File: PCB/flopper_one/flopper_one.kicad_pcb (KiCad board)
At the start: 2 copper layers, 76.8 x 63 mm, 24 parts, among them J1 To PN532 ->, J2 <- ST7789, Q1 2N2219, SW1 SW_Omron_B3FS, SW2 SW_Omron_B3FS, SW3 SW_Omron_B3FS, SW4 SW_Omron_B3FS, SW5 SW_Omron_B3FS, SW6 SW_SPST, U1 TP4056-42-ESOP8, U4 hw-045

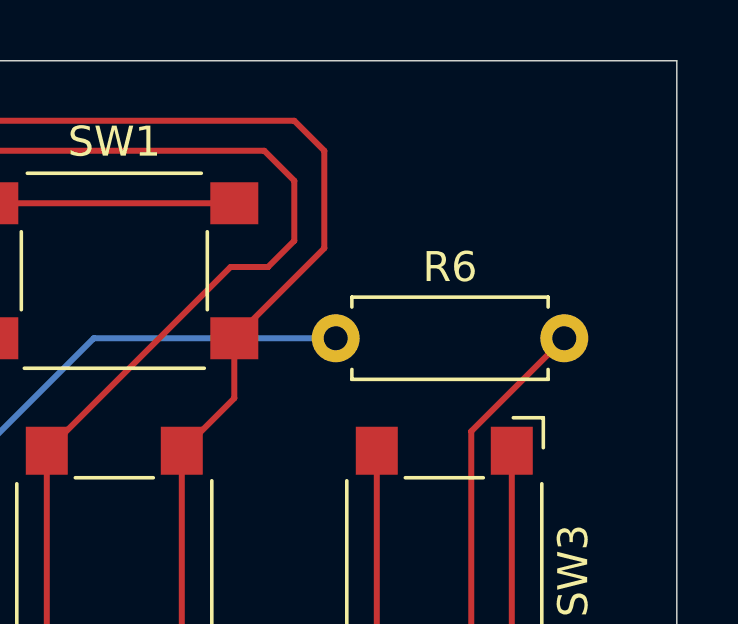
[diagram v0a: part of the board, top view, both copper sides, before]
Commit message: flip r6
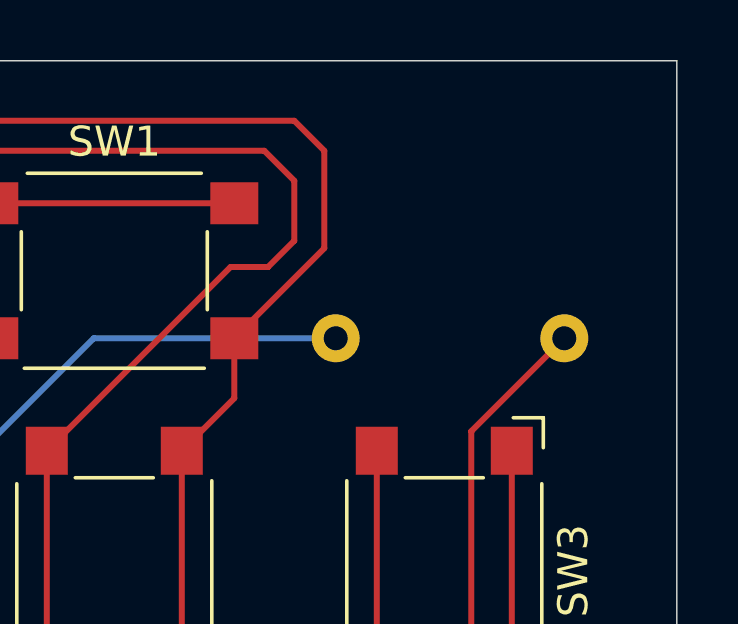
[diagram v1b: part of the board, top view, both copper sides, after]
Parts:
- R6: moved to B.Cu
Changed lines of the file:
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@@
-		)
-	)
-	(footprint "Resistor_THT:R_Axial_DIN0207_L6.3mm_D2.5mm_P7.62mm_Horizontal"
-		(layer "F.Cu")
-		(at 98.38 33.5)
-		(descr "Resistor, Axial_DIN0207 series, Axial, Horizontal, pin pitch=7.62mm, 0.25W = 1/4W, length*diameter=6.3*2.5mm^2, http://cdn-reichelt.de/documents/datenblatt/B400/1_4W%23YAG.pdf")
-		(tags "Resistor Axial_DIN0207 series Axial Horizontal pin pitch 7.62mm 0.25W = 1/4W length 6.3mm diameter 2.5mm")
-		(property "Reference" "R6"
-			(at 3.81 -2.37 0)
-			(layer "F.SilkS")
-			(effects
-				(font
-					(size 1 1)
-					(thickness 0.15)
-				)
-			)
-		)
-		(property "Value" "0.4Ω"
-			(at 3.81 2.37 0)
-			(layer "F.Fab")
-			(effects
-				(font
-					(size 1 1)
-					(thickness 0.15)
-				)
-			)
-		)
-		(property "Datasheet" "~"
-			(at 0 0 0)
-			(layer "F.Fab")
-			(hide yes)
-			(effects
-				(font
-					(size 1.27 1.27)
-					(thickness 0.15)
-				)
-			)
-		)
-		(property "Description" "Resistor, US symbol"
-			(at 0 0 0)
-			(layer "F.Fab")
-			(hide yes)
-			(effects
-				(font
-					(size 1.27 1.27)
-					(thickness 0.15)
-				)
-			)
-		)
-		(property ki_fp_filters "R_*")
-		(sheetname "/")
-		(sheetfile "flopper_one.kicad_sch")
-		(attr through_hole)
-		(fp_line
-			(start 0.54 -1.37)
-			(end 7.08 -1.37)
-			(stroke
-				(width 0.12)
-				(type solid)
-			)
-			(layer "F.SilkS")
-		)
-		(fp_line
-			(start 0.54 -1.04)
-			(end 0.54 -1.37)
-			(stroke
-				(width 0.12)
-				(type solid)
-			)
-			(layer "F.SilkS")
-		)
-		(fp_line
-			(start 0.54 1.04)
-			(end 0.54 1.37)
-			(stroke
-				(width 0.12)
-				(type solid)
-			)
-			(layer "F.SilkS")
-		)
-		(fp_line
-			(start 0.54 1.37)
-			(end 7.08 1.37)
-			(stroke
-				(width 0.12)
-				(type solid)
-			)
-			(layer "F.SilkS")
-		)
-		(fp_line
-			(start 7.08 -1.37)
-			(end 7.08 -1.04)
-			(stroke
-				(width 0.12)
-				(type solid)
-			)
-			(layer "F.SilkS")
-		)
-		(fp_line
-			(start 7.08 1.37)
-			(end 7.08 1.04)
-			(stroke
-				(width 0.12)
-				(type solid)
-			)
-			(layer "F.SilkS")
-		)
-		(fp_rect
-			(start -1.05 -1.5)
-			(end 8.67 1.5)
-			(stroke
-				(width 0.05)
-				(type solid)
-			)
-			(fill no)
-			(layer "F.CrtYd")
-		)
-		(fp_line
-			(start 0 0)
-			(end 0.66 0)
-			(stroke
-				(width 0.1)
-				(type solid)
-			)
-			(layer "F.Fab")
-		)
-		(fp_line
-			(start 7.62 0)
-			(end 6.96 0)
-			(stroke
-				(width 0.1)
-				(type solid)
-			)
-			(layer "F.Fab")
-		)
-		(fp_rect
-			(start 0.66 -1.25)
-			(end 6.96 1.25)
-			(stroke
-				(width 0.1)
-				(type solid)
-			)
-			(fill no)
-			(layer "F.Fab")
-		)
-		(fp_text user "${REFERENCE}"
-			(at 3.81 0 0)
-			(layer "F.Fab")
-			(effects
-				(font
-					(size 1 1)
-					(thickness 0.15)
-				)
-			)
-		)
-		(pad "1" thru_hole circle
-			(at 0 0)
-			(size 1.6 1.6)
-			(drill 0.8)
-			(layers "*.Cu" "*.Mask")
-			(remove_unused_layers no)
-			(net 40 "/VIN")
-			(pintype "passive")
-		)
-		(pad "2" thru_hole circle
-			(at 7.62 0)
-			(size 1.6 1.6)
-			(drill 0.8)
-			(layers "*.Cu" "*.Mask")
-			(remove_unused_layers no)
-			(net 42 "Net-(D2-A)")
-			(pintype "passive")
-		)
-		(embedded_fonts no)
-		(model "${KICAD9_3DMODEL_DIR}/Resistor_THT.3dshapes/R_Axial_DIN0207_L6.3mm_D2.5mm_P7.62mm_Horizontal.step"
-			(offset
-				(xyz 0 0 0)
-			)
-			(scale
-				(xyz 1 1 1)
-			)
-			(rotate
-				(xyz 0 0 0)
-			)
 		)
 	)
@@
 			(offset
 				(xyz 0 0 0)
+			)
+			(scale
+				(xyz 1 1 1)
+			)
+			(rotate
+				(xyz 0 0 0)
+			)
+		)
+	)
+	(footprint "Resistor_THT:R_Axial_DIN0207_L6.3mm_D2.5mm_P7.62mm_Horizontal"
+		(layer "B.Cu")
+		(at 98.38 33.5)
+		(descr "Resistor, Axial_DIN0207 series, Axial, Horizontal, pin pitch=7.62mm, 0.25W = 1/4W, length*diameter=6.3*2.5mm^2, http://cdn-reichelt.de/documents/datenblatt/B400/1_4W%23YAG.pdf")
+		(tags "Resistor Axial_DIN0207 series Axial Horizontal pin pitch 7.62mm 0.25W = 1/4W length 6.3mm diameter 2.5mm")
+		(property "Reference" "R6"
+			(at 3.81 2.37 0)
+			(layer "B.SilkS")
+			(effects
+				(font
+					(size 1 1)
+					(thickness 0.15)
+				)
+				(justify mirror)
+			)
+		)
+		(property "Value" "0.4Ω"
+			(at 3.81 -2.37 0)
+			(layer "B.Fab")
+			(effects
+				(font
+					(size 1 1)
+					(thickness 0.15)
+				)
+				(justify mirror)
+			)
+		)
+		(property "Datasheet" "~"
+			(at 0 0 0)
+			(layer "B.Fab")
+			(hide yes)
+			(effects
+				(font
+					(size 1.27 1.27)
+					(thickness 0.15)
+				)
+				(justify mirror)
+			)
+		)
+		(property "Description" "Resistor, US symbol"
+			(at 0 0 0)
+			(layer "B.Fab")
+			(hide yes)
+			(effects
+				(font
+					(size 1.27 1.27)
+					(thickness 0.15)
+				)
+				(justify mirror)
+			)
+		)
+		(property ki_fp_filters "R_*")
+		(sheetname "/")
+		(sheetfile "flopper_one.kicad_sch")
+		(attr through_hole)
+		(fp_line
+			(start 0.54 -1.37)
+			(end 7.08 -1.37)
+			(stroke
+				(width 0.12)
+				(type solid)
+			)
+			(layer "B.SilkS")
+		)
+		(fp_line
+			(start 0.54 -1.04)
+			(end 0.54 -1.37)
+			(stroke
+				(width 0.12)
+				(type solid)
+			)
+			(layer "B.SilkS")
+		)
+		(fp_line
+			(start 0.54 1.04)
+			(end 0.54 1.37)
+			(stroke
+				(width 0.12)
+				(type solid)
+			)
+			(layer "B.SilkS")
+		)
+		(fp_line
+			(start 0.54 1.37)
+			(end 7.08 1.37)
+			(stroke
+				(width 0.12)
+				(type solid)
+			)
+			(layer "B.SilkS")
+		)
+		(fp_line
+			(start 7.08 -1.37)
+			(end 7.08 -1.04)
+			(stroke
+				(width 0.12)
+				(type solid)
+			)
+			(layer "B.SilkS")
+		)
+		(fp_line
+			(start 7.08 1.37)
+			(end 7.08 1.04)
+			(stroke
+				(width 0.12)
+				(type solid)
+			)
+			(layer "B.SilkS")
+		)
+		(fp_rect
+			(start -1.05 1.5)
+			(end 8.67 -1.5)
+			(stroke
+				(width 0.05)
+				(type solid)
+			)
+			(fill no)
+			(layer "B.CrtYd")
+		)
+		(fp_line
+			(start 0 0)
+			(end 0.66 0)
+			(stroke
+				(width 0.1)
+				(type solid)
+			)
+			(layer "B.Fab")
+		)
+		(fp_line
+			(start 7.62 0)
+			(end 6.96 0)
+			(stroke
+				(width 0.1)
+				(type solid)
+			)
+			(layer "B.Fab")
+		)
+		(fp_rect
+			(start 0.66 1.25)
+			(end 6.96 -1.25)
+			(stroke
+				(width 0.1)
+				(type solid)
+			)
+			(fill no)
+			(layer "B.Fab")
+		)
+		(fp_text user "${REFERENCE}"
+			(at 3.81 0 0)
+			(layer "B.Fab")
+			(effects
+				(font
+					(size 1 1)
+					(thickness 0.15)
+				)
+				(justify mirror)
+			)
+		)
+		(pad "1" thru_hole circle
+			(at 0 0)
+			(size 1.6 1.6)
+			(drill 0.8)
+			(layers "*.Cu" "*.Mask")
+			(remove_unused_layers no)
+			(net 40 "/VIN")
+			(pintype "passive")
+		)
+		(pad "2" thru_hole circle
+			(at 7.62 0)
+			(size 1.6 1.6)
+			(drill 0.8)
+			(layers "*.Cu" "*.Mask")
+			(remove_unused_layers no)
+			(net 42 "Net-(D2-A)")
+			(pintype "passive")
+		)
+		(embedded_fonts no)
+		(model "${KICAD9_3DMODEL_DIR}/Resistor_THT.3dshapes/R_Axial_DIN0207_L6.3mm_D2.5mm_P7.62mm_Horizontal.step"
+			(offset
+				(xyz 0 0 0)
